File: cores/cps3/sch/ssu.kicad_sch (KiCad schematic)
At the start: 1 part

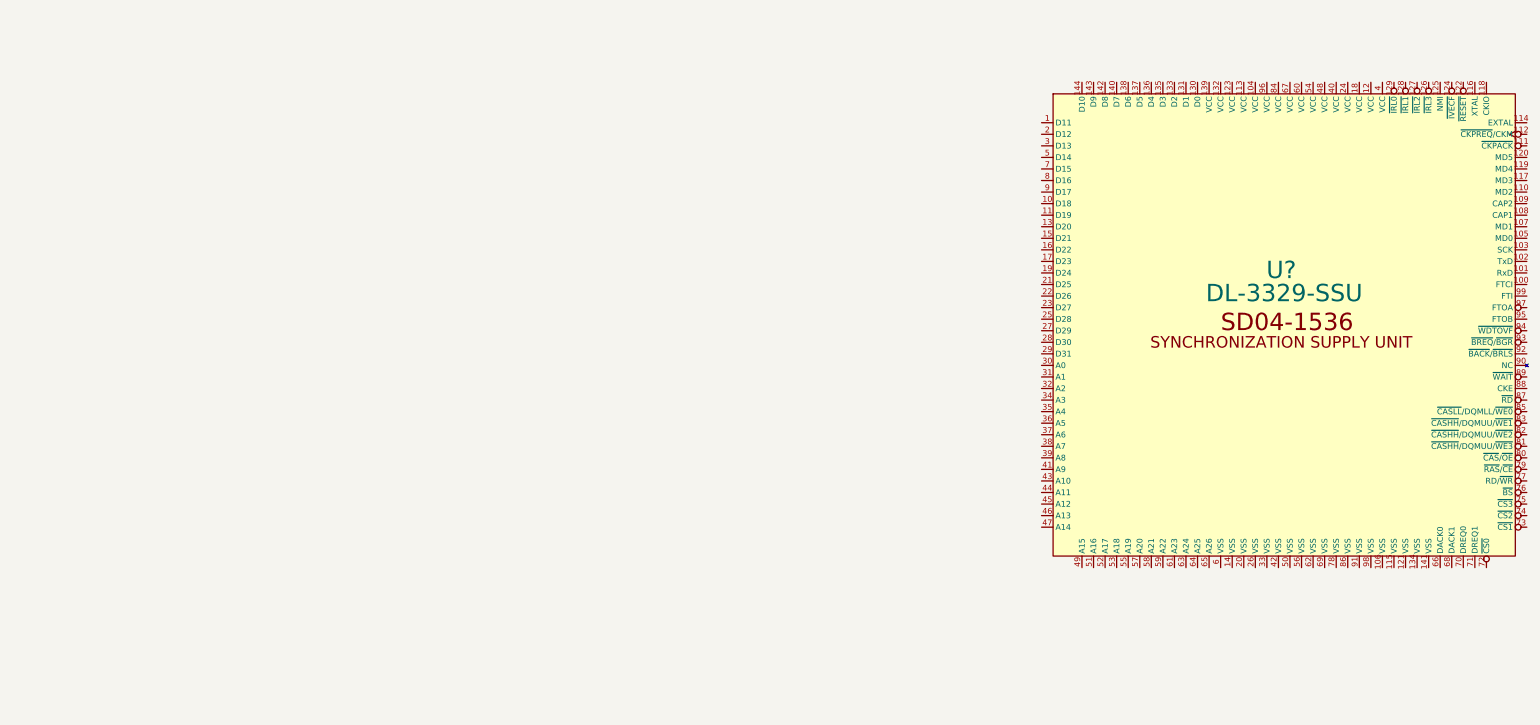
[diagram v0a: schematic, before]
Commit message: ssu_gll
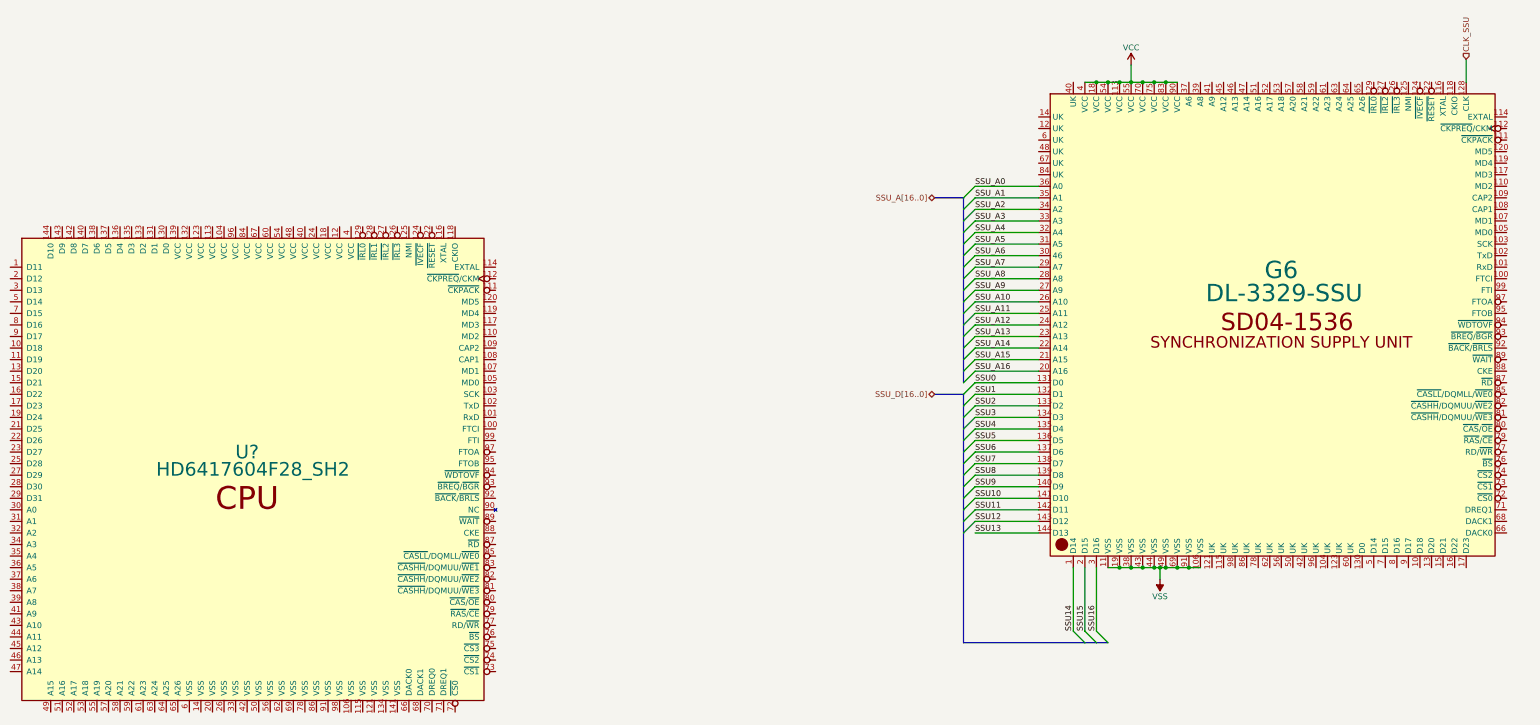
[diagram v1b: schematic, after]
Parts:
- added U?: HD6417604F28_SH2, symbol arcade:HD6417604F28_SH2
- gave numbers to parts that had none: 1
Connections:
- net SSU14: now reaches G6.1 (D14)
- net VSS: now reaches G6.106 (VSS)
- net VSS: now also G6.11 (VSS), G6.19 (VSS), G6.38 (VSS), G6.43 (VSS), G6.44 (VSS), G6.49 (VSS), G6.69 (VSS), G6.91 (VSS)
- net VCC: now reaches G6.113 (VCC)
- net VCC: now also G6.18 (VCC), G6.4 (VCC), G6.54 (VCC), G6.55 (VCC), G6.70 (VCC), G6.75 (VCC), G6.83 (VCC), G6.90 (VCC)
- net CLK_SSU: now reaches G6.128 (CLK)
- net SSU0: now reaches G6.131 (D0)
- net SSU1: now reaches G6.132 (D1)
- net SSU2: now reaches G6.133 (D2)
- net SSU3: now reaches G6.134 (D3)
- net SSU4: now reaches G6.135 (D4)
- net SSU5: now reaches G6.136 (D5)
- net SSU6: now reaches G6.137 (D6)
- net SSU7: now reaches G6.138 (D7)
- net SSU8: now reaches G6.139 (D8)
- net SSU9: now reaches G6.140 (D9)
- net SSU10: now reaches G6.141 (D10)
- net SSU11: now reaches G6.142 (D11)
- net SSU12: now reaches G6.143 (D12)
- net SSU13: now reaches G6.144 (D13)
- net SSU15: now reaches G6.2 (D15)
- net SSU_A16: now reaches G6.20 (A16)
- net SSU_A15: now reaches G6.21 (A15)
- net SSU_A14: now reaches G6.22 (A14)
- net SSU_A13: now reaches G6.23 (A13)
- net SSU_A12: now reaches G6.24 (A12)
- net SSU_A11: now reaches G6.25 (A11)
- net SSU_A10: now reaches G6.26 (A10)
- net SSU_A9: now reaches G6.27 (A9)
- net SSU_A8: now reaches G6.28 (A8)
- net SSU_A7: now reaches G6.29 (A7)
- net SSU16: now reaches G6.3 (D16)
- net SSU_A6: now reaches G6.30 (46)
- net SSU_A5: now reaches G6.31 (A5)
- net SSU_A4: now reaches G6.32 (A4)
- net SSU_A3: now reaches G6.33 (A3)
- net SSU_A2: now reaches G6.34 (A2)
- net SSU_A1: now reaches G6.35 (A1)
- net SSU_A0: now reaches G6.36 (A0)
